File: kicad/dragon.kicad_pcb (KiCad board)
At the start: 2 copper layers, 60 x 60 mm, 4 parts

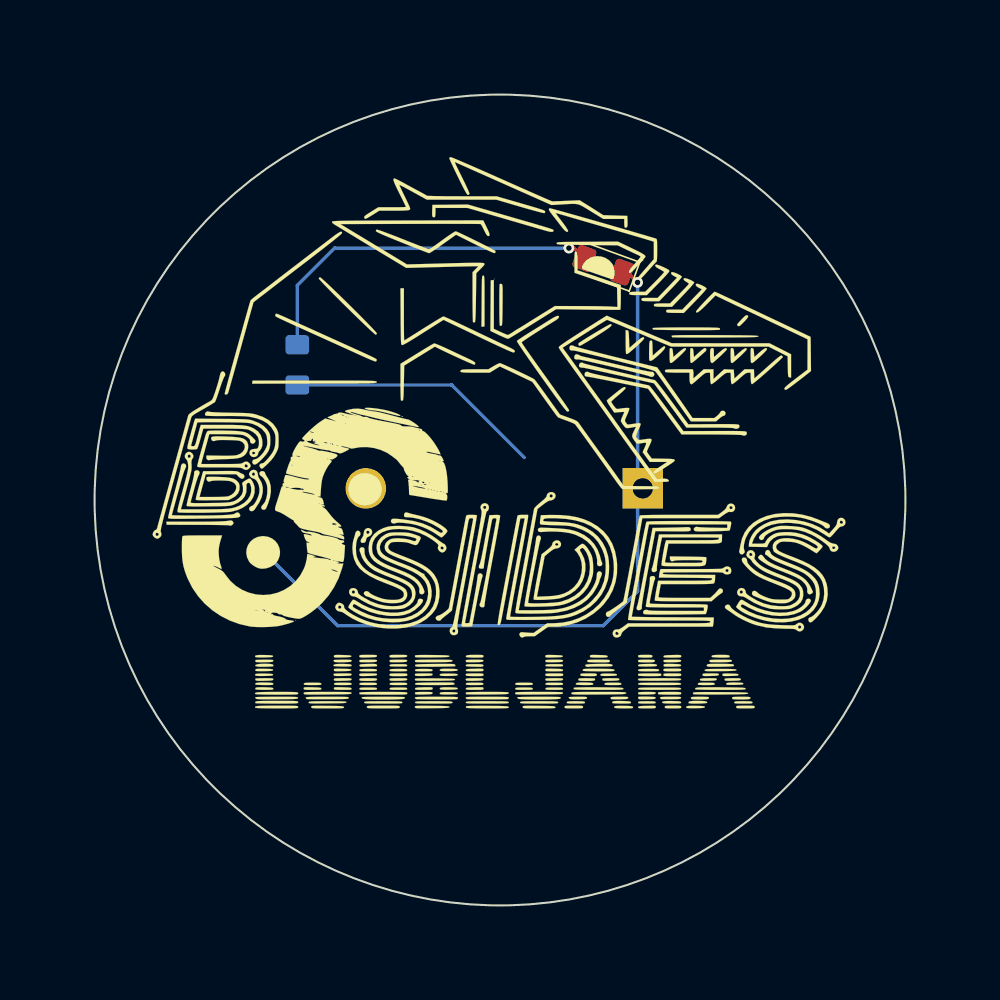
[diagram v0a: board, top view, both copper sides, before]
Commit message: Add hole
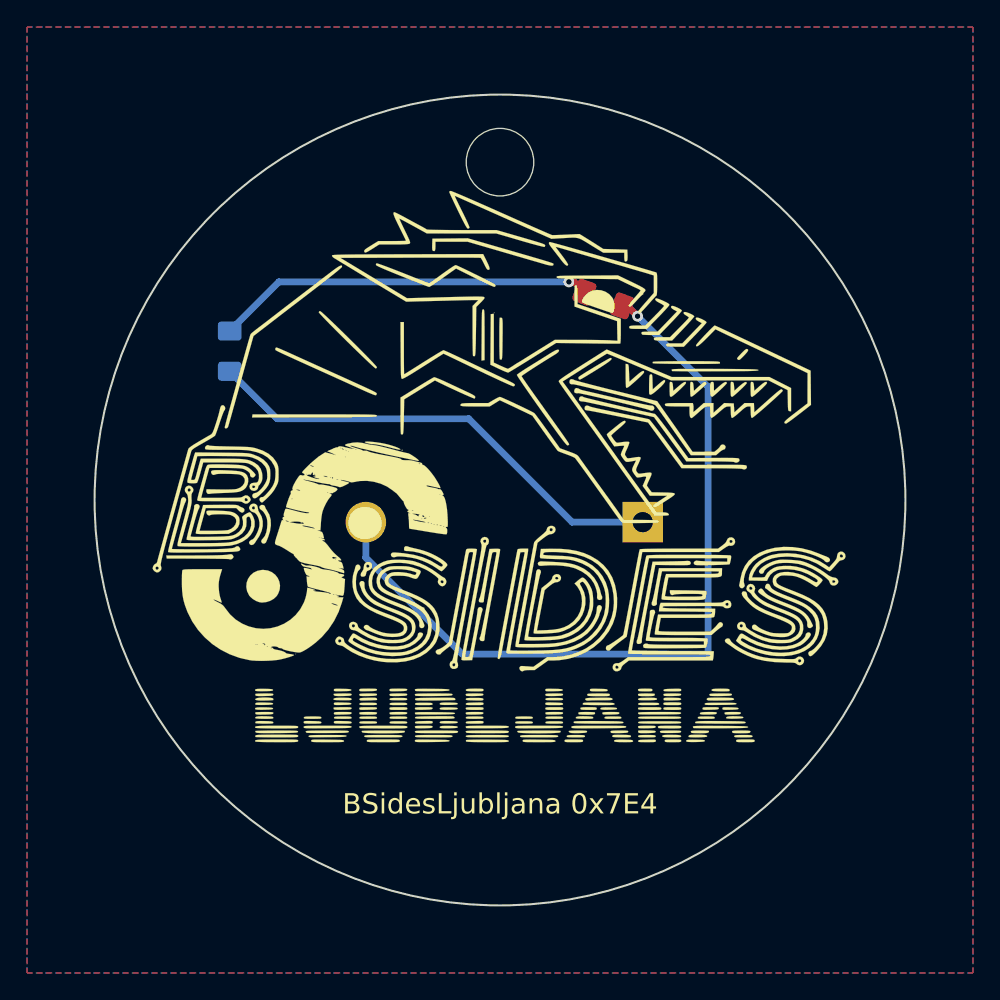
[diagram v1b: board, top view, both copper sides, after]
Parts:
- added REF**: MountingHole_5mm, dragon:MountingHole_5mm, F.Cu at (160.0, 80.0)
- D1: footprint LED_SMD:LED_1206_3216Metric_Pad1.42x1.75mm_HandSolder -> dragon:LED_1206_3216Metric_Pad1.42x1.75mm_HandSolder_dragon
- moved R1 5.10 mm to (140.0, 94.0)
- moved BT1 2.50 mm to (170.6, 106.6)
- moved D1 2.50 mm to (167.6, 90.1)
- moved G*** 2.50 mm to (160.0, 102.5)
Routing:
- net Net-(BT1-Pad1): track 19.0 -> 35.2 mm
- net Net-(BT1-Pad2): track 55.3 -> 60.4 mm
- net Net-(D1-Pad2): track 27.1 -> 28.1 mm
- added copper zone on B.Cu, net Net-(BT1-Pad2)
- added copper zone on F.Cu, net Net-(D1-Pad2)
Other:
- net class Default: trace_width 0.25 -> 0.5
- board text added: "BSidesLjubljana 0x7E4"

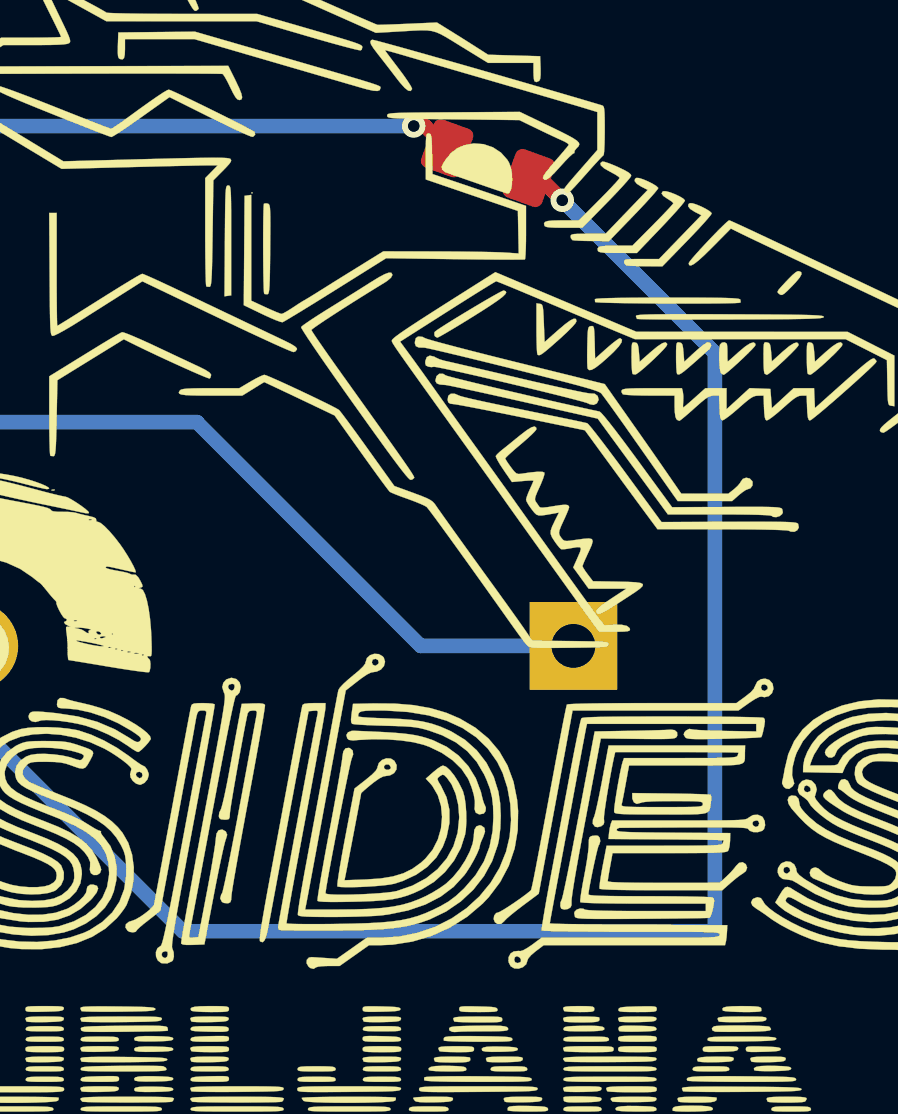
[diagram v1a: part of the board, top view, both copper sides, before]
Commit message: Final
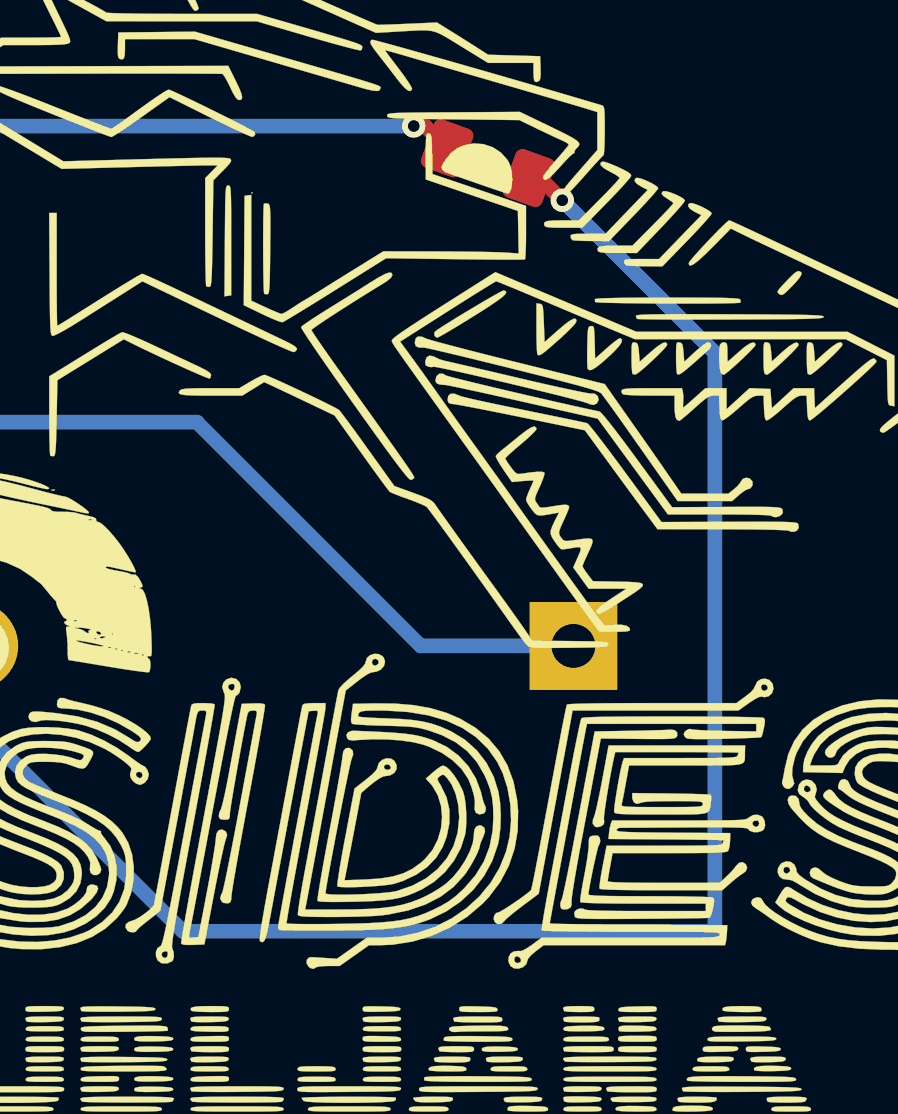
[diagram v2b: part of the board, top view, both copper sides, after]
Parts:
- BT1: footprint Battery:BatteryHolder_Keystone_106_1x20mm -> dragon:BatteryHolder_Keystone_106_1x20mm
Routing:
- net Net-(BT1-Pad2): track 60.4 -> 59.5 mm
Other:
- board text added: "aGVyZSBiZSBkcmFnb25z"
